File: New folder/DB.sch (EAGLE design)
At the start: 20 parts, among them J1 TYPE-C-31-M-12, U3 LTC4054, U6 DW01A, U7 FS8205, X2 BM06B-SRSS-TB

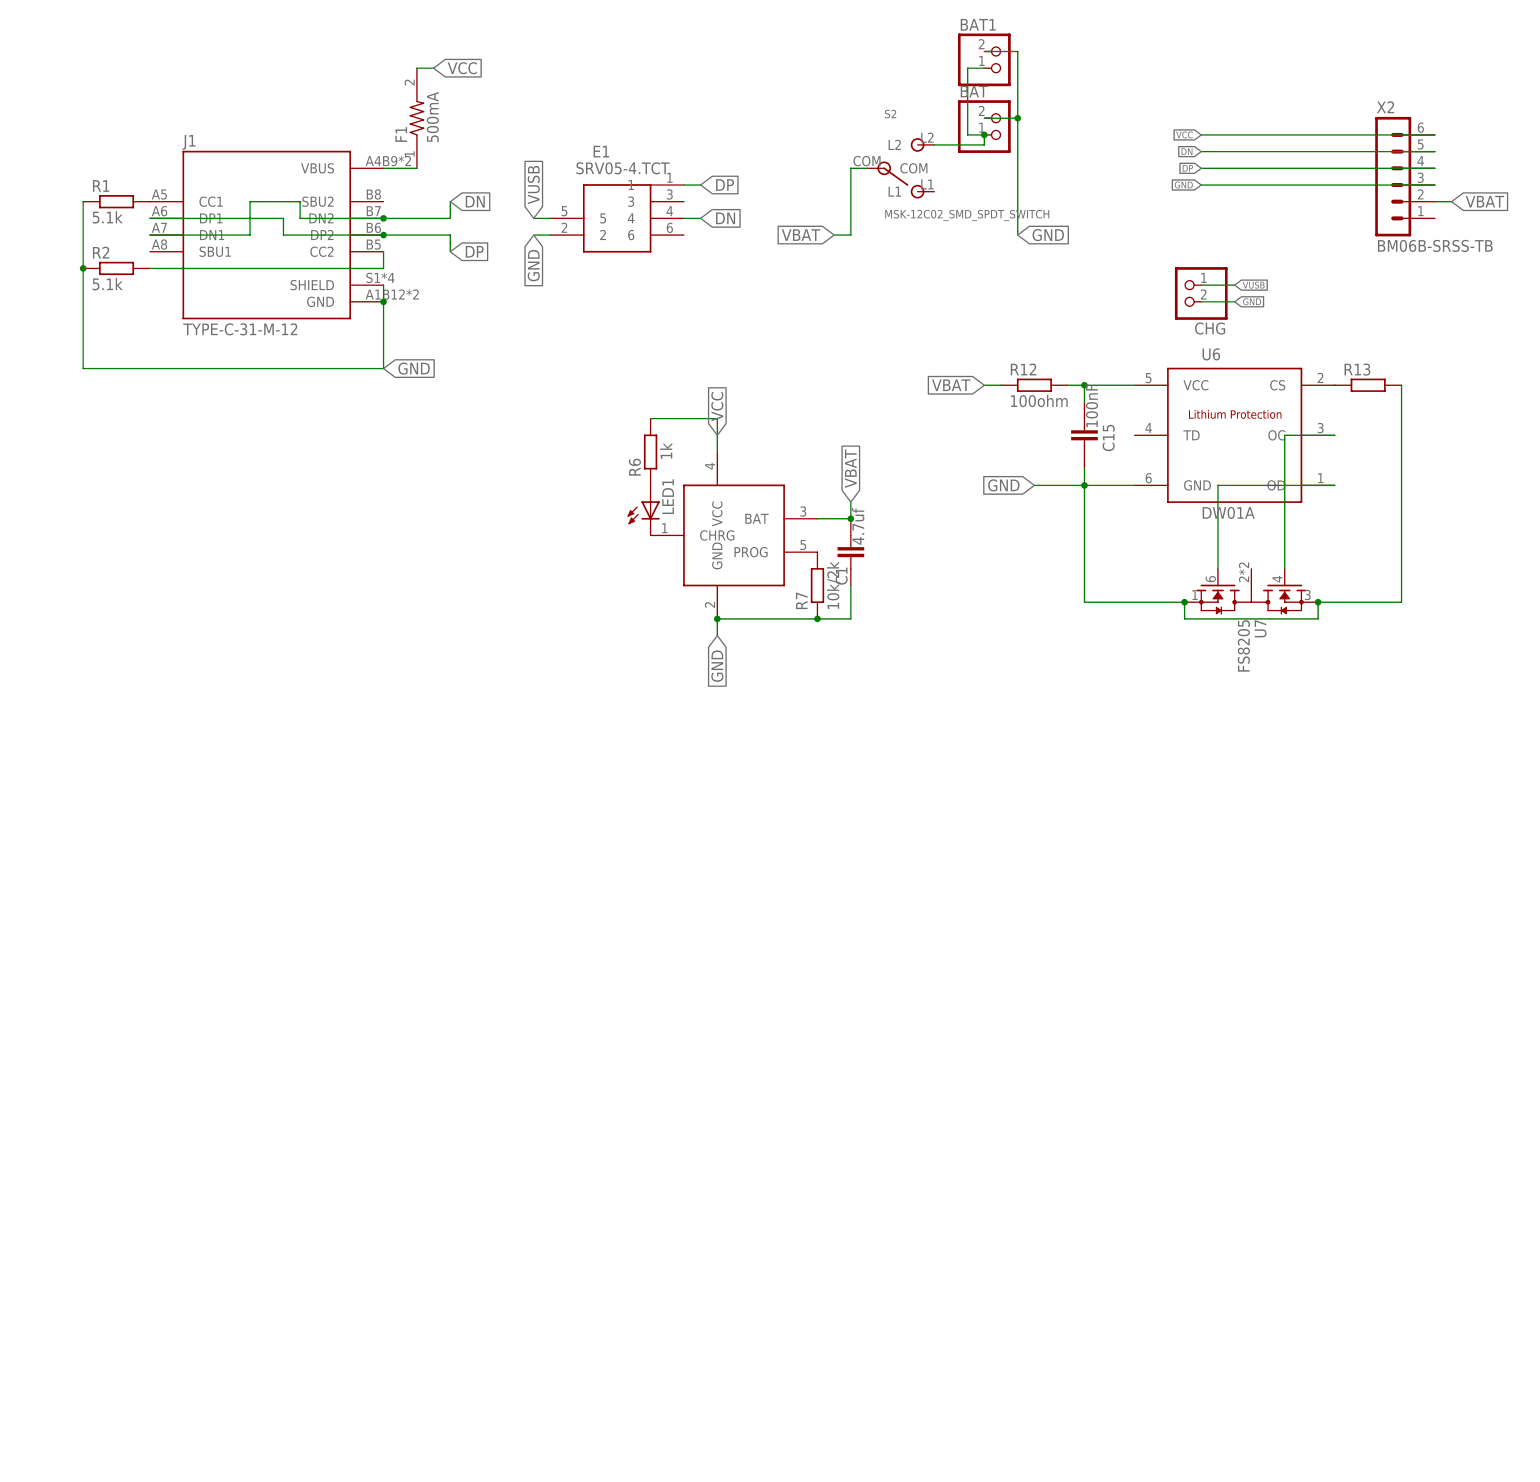
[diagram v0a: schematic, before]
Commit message: add
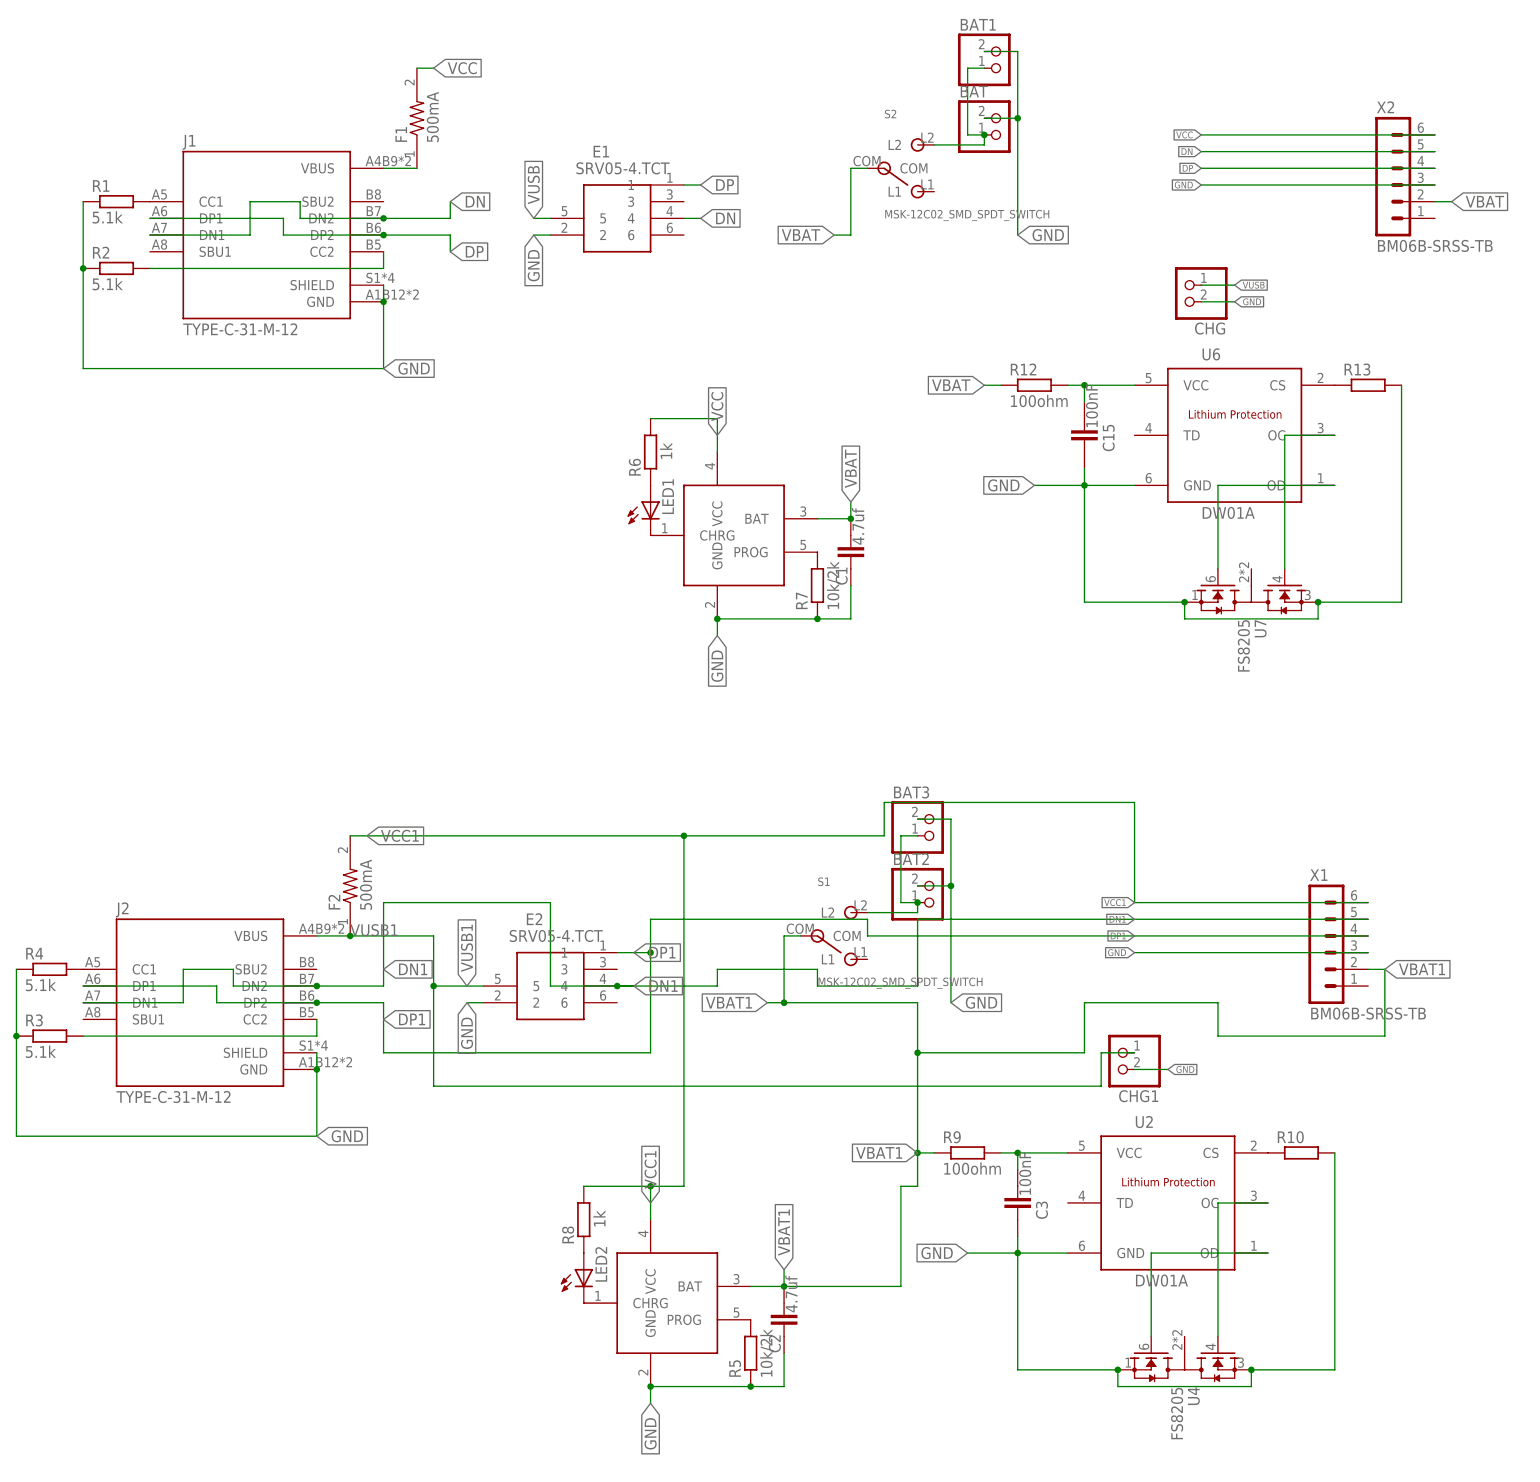
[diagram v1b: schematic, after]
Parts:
- added BAT2, BAT3, CHG1: (no value), adafruit:JST_2PIN-THM-RA
- added C2: 4.7uf, Components:CAPACITOR-C0805
- added C3: 100nF, Components:CAPACITOR-C0805
- added E2: SRV05-4.TCT, SRV05-4.TCT:SRV05-4.TCT
- added F2: 500mA, fuse:0ZCJ0075AF2E
- added J2: TYPE-C-31-M-12, TYPE-C-31-M-12:TYPE-C-31-M-12
- added LED2: (no value), adafruit:LEDCHIPLED_1206
- added R10: (no value), Components:RESISTOR-0805
- added R3, R4: 5.1k, Components:RESISTOR-0805
- added R5: 10k/2k, Components:RESISTOR-0805
- added R8: 1k, Components:RESISTOR-0805
- added R9: 100ohm, Components:RESISTOR-0805
- added S1: MSK-12C02_SMD_SPDT_SWITCH, MSK-12C02 SMD Micro Slider Switch SPDT:MSK-12C02_SMD_SPDT_SWITCH
- added U1: LTC4054, LTC4054:LTC4054
- added U2: DW01A, DW01A:DW01A
- added U4: FS8205, FS8205:FS8205
- added X1: BM06B-SRSS-TB, con-JST SH:BM06B-SRSS-TB
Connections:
- new net DN1: E2.4, J2.DN1, J2.DN2, X1.5
- new net DP1: E2.1, J2.DP1, J2.DP2, X1.4
- new net N$41: J2.CC1, R4.2
- new net N$42: J2.CC2, R3.2
- new net N$43: R5.2, U1.PROG
- new net N$44: LED2.C, U1.CHRG
- new net N$45: LED2.A, R8.1
- new net N$46: BAT2.2, BAT3.2, S1.L2
- new net N$47: C3.2, R9.2, U2.VCC
- new net N$48: R10.1, U2.CS
- new net N$49: U2.OD, U4.G1
- new net N$50: U2.OC, U4.G2
- new net VBAT1: C2.2, R9.1, S1.COM, U1.BAT, X1.2
- new net VCC1: F2.2, R8.2, U1.VCC, X1.6
- new net VUSB1: CHG1.2, E2.5, F2.1, J2.VBUS
- net GND: now also BAT2.1, BAT3.1, C2.1, C3.1, CHG1.1, E2.2, J2.GND, J2.SHIELD, R10.2, R3.1, R4.1, R5.1, U1.GND, U2.GND, U4.S1, U4.S2, X1.3
